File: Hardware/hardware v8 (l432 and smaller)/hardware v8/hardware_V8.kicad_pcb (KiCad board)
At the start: 6 copper layers, 21.6 x 20.8 mm, 69 parts, among them IC1 TPS22960RSER, IC4 MAX-M10S-00B, IC5 LTC4065EDC#TRMPBF, IC6 W25Q128JVPIQ, J1 USB4720-03-A, J2 503548-0622, J3 OLED, SW4 boot, U1 STM32L432KCUx, U2 ldln025pu, U3 146235-0001

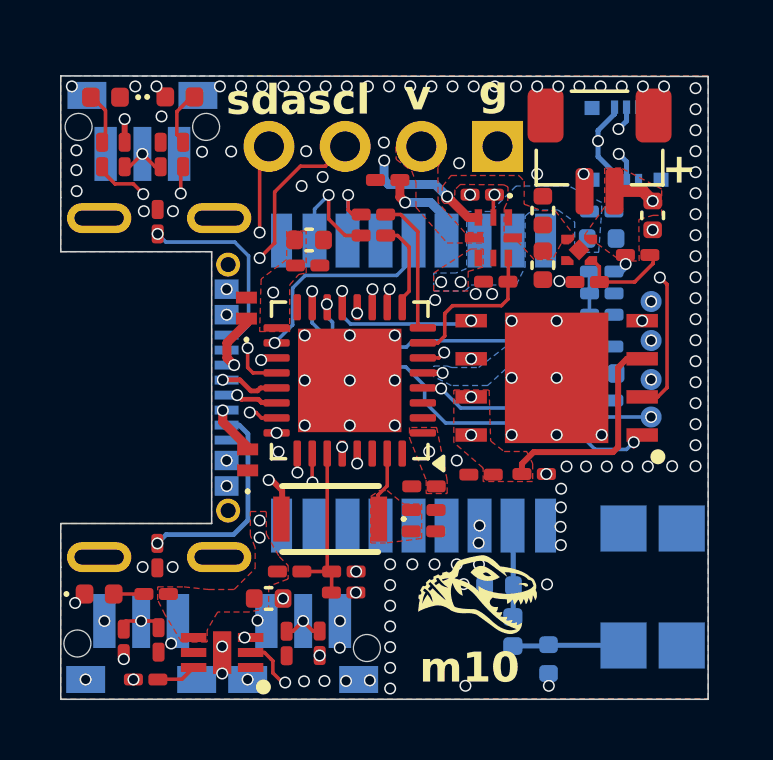
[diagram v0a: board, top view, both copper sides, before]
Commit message: up
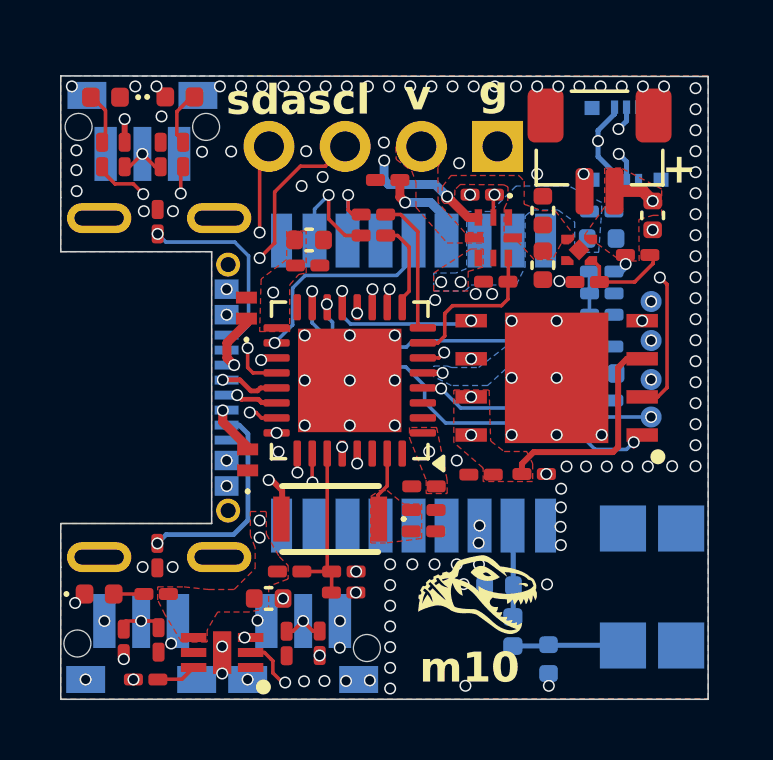
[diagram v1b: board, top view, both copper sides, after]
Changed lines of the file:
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@@
 		)
 		(embedded_fonts no)
-		(model "${KICAD9_3DMODEL_DIR}/Connector_JST.3dshapes/JST_SH_BM02B-SRSS-TB_1x02-1MP_P1.00mm_Vertical.step"
-			(offset
-				(xyz 0 0 0)
-			)
-			(scale
-				(xyz 1 1 1)
-			)
-			(rotate
-				(xyz 0 0 0)
-			)
-		)
 	)
 	(footprint "Capacitor_SMD:C_0201_0603Metric_Pad0.64x0.40mm_HandSolder"
@@
 	(footprint "samacsys2:146235-0001"
 		(layer "B.Cu")
-		(at 131.4 104.315 90)
+		(at 131.38 104.315 90)
 		(descr "146235-0001")
 		(tags "Undefined or Miscellaneous")
@@
 		)
 		(embedded_fonts no)
-		(model "${KICAD9_3DMODEL_DIR}/Connector_PinSocket_2.54mm.3dshapes/PinSocket_1x04_P2.54mm_Vertical.step"
-			(offset
-				(xyz 0 0 0)
-			)
-			(scale
-				(xyz 1 1 1)
-			)
-			(rotate
-				(xyz 0 0 0)
-			)
-		)
 	)
 	(footprint "samacsys:MAXM10S00B"
@@
 	)
 	(segment
-		(start 130.425 106.26)
-		(end 130.43 106.265)
+		(start 130.405 106.26)
+		(end 130.41 106.265)
 		(width 0.1693)
 		(layer "B.Cu")
@@
 	)
 	(segment
-		(start 127.95 106.26)
-		(end 130.425 106.26)
+		(start 126.74 106.285)
+		(end 126.75 106.285)
 		(width 0.1693)
 		(layer "B.Cu")
@@
 	)
 	(segment
-		(start 126.74 106.285)
-		(end 126.75 106.285)
+		(start 127.95 106.26)
+		(end 130.405 106.26)
 		(width 0.1693)
 		(layer "B.Cu")
